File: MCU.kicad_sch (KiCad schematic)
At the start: 48 parts, among them IC3 TCAN330DCNT, J1 BM04B-GHS-TBT_LF__SN__N_, J2 Conn_01x04_Pin, J3 USB_C_Receptacle_USB2.0_16P, J4 BM04B-GHS-TBT_LF__SN__N_, J5 Conn_01x02_Socket, SW1 SW_SPDT, SW2 SW_SPDT, U2 STM32G431CBU6, U3 ME6211C33M5, Y1 ECS-80-20-5PX-TR

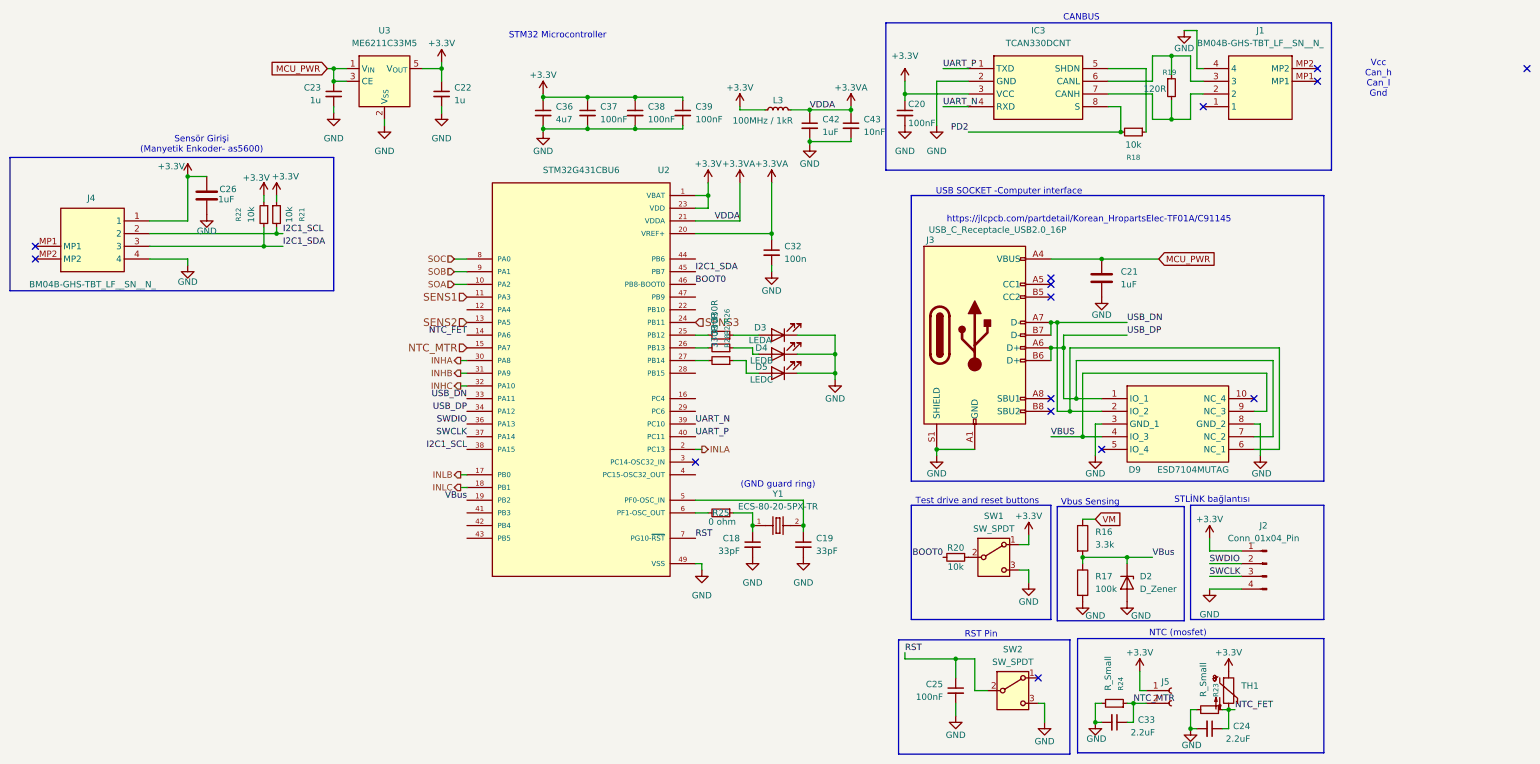
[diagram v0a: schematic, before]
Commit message: all nıght 4/12
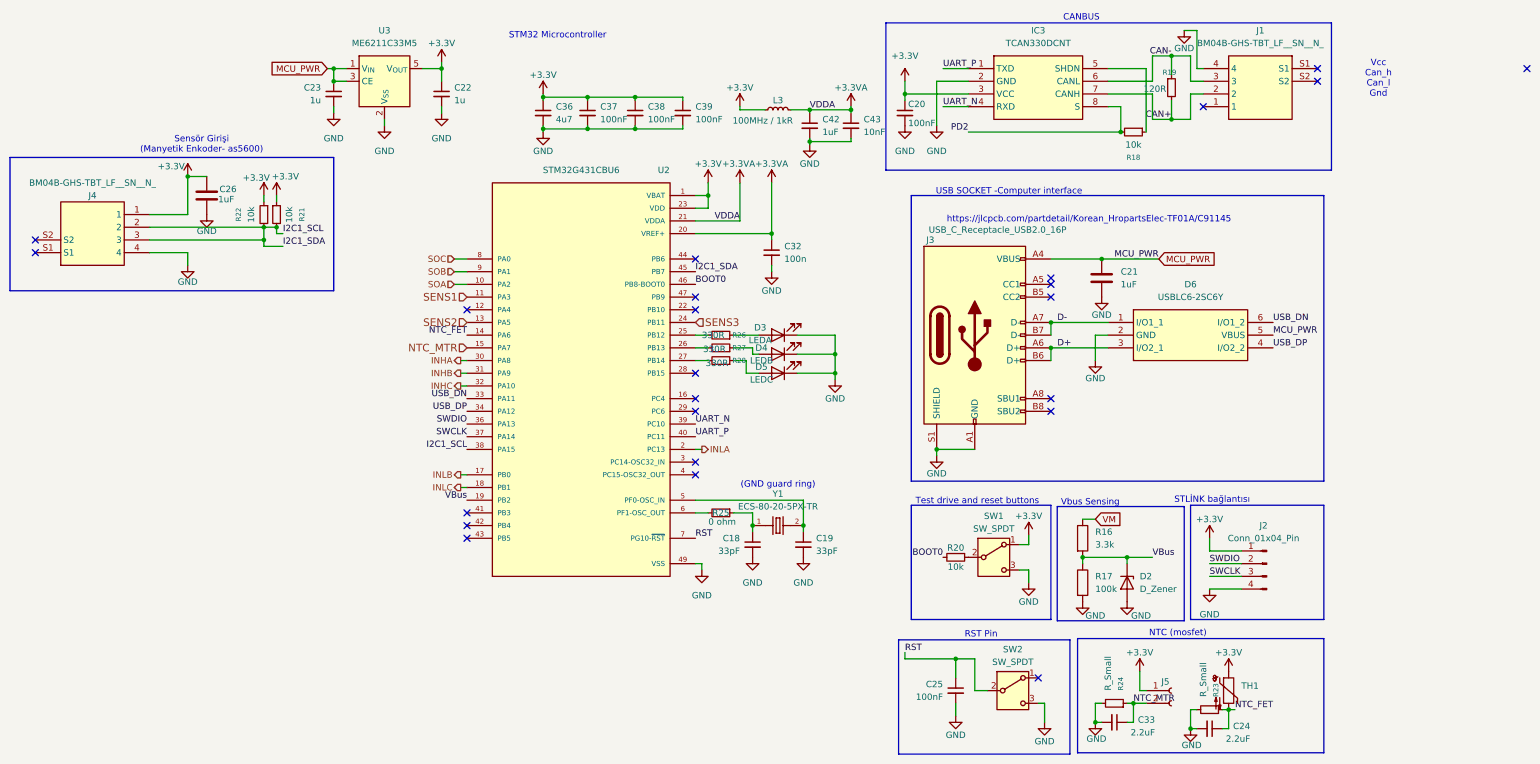
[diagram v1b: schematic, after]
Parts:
- removed D9: ESD7104MUTAG, LIB_ESD7104MUTAG:ESD8104MUTAG, symbol ESD7104MUTAG:ESD7104MUTAG
- added D6: USBLC6-2SC6Y, SOT95P280X145-6N, symbol USBLC6-2SC6Y:USBLC6-2SC6Y
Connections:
- net I2C1_SDA is gone; now on net I2C1_SCL: J4.3, R22.2, U2.45 (PB7)
- net GND: now also D6.2 (GND)
- net MCU_PWR: now also D6.5 (VBUS)
- net USB_DN: now also D6.6 (I/O1_2); no longer J3.A7 (D-), J3.B7 (D-)
- net USB_DP: now also D6.4 (I/O2_2); no longer J3.A6 (D+), J3.B6 (D+)
- net CAN-: now reaches IC3.6 (CANL), J1.3, R19.1
- net CAN+: now reaches IC3.7 (CANH), J1.2, R19.2
- new net D+: D6.3 (I/O2_1), J3.A6 (D+), J3.B6 (D+)
- new net D-: D6.1 (I/O1_1), J3.A7 (D-), J3.B7 (D-)
- no-connect marks 15 -> 24
